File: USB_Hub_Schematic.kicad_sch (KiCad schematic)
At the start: 107 parts, among them J1 USB-C, J2 USB-A, U1 USB2517 Chip, U10 TP, U11 TP, U12 TP, U13 TP, U14 TP, U15 TP, U16 TPS25821, U17 TPS25821, U18 TP, U19 TP, U2 3.3V CONV, U3 MUX, U4 USB to microSD, U5 24AA02, U7 TPS2052B, U9 TP, X3 24MHz Osc

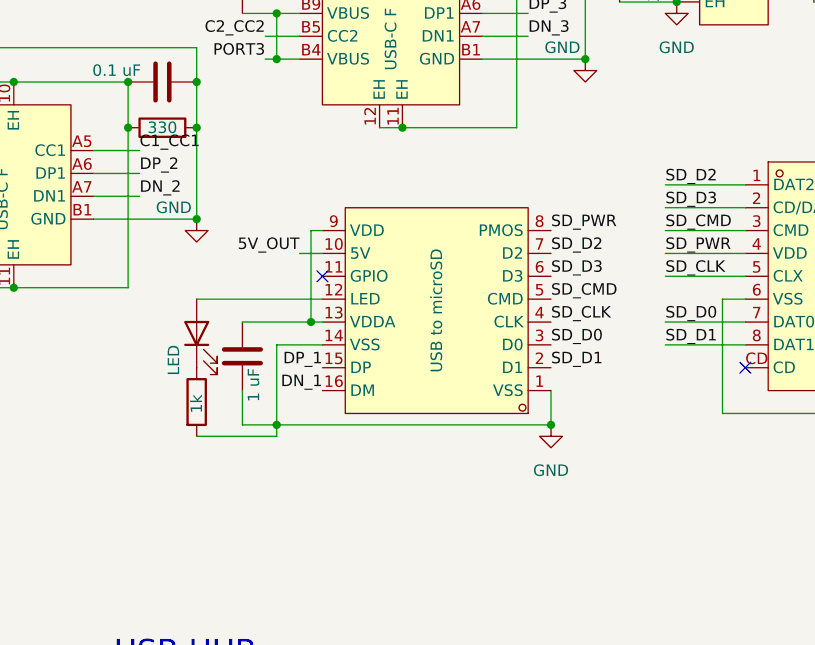
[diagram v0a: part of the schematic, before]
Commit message: PCBWay Order Sent
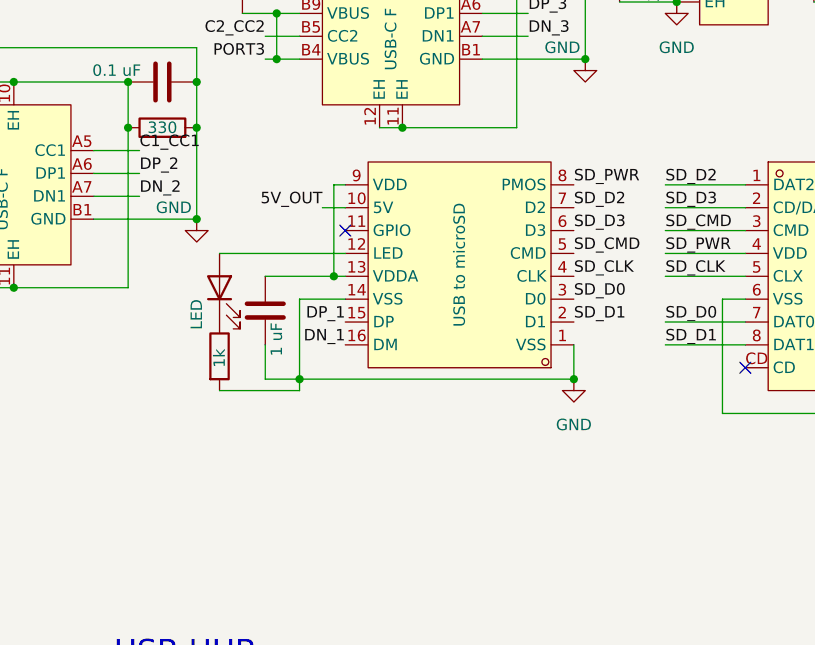
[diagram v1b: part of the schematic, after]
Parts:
- C1, C20, C22, C31, C35, C4, C5: LCSC Part (none) -> C15849
- C12, C13, C17, C3, C33, C38, C39: LCSC Part (none) -> C16780
- C18, C2, C23, C24, C25, C26, C29, C32, C36, C37, C40, C41, C42, C44, C9: LCSC Part (none) -> C1525
- C19, C21, C30, C48: LCSC Part (none) -> C342635
- C28: LCSC Part (none) -> C19666
- C43, C45: LCSC Part (none) -> C15008
- D10, D13, D14, D15, D2: LCSC Part (none) -> C2290
- D11, D12, D16, D17: LCSC Part (none) -> C2286
- R1, R16, R2, R34, R47, R49, R51, R54, R56: LCSC Part (none) -> C25803
- R10, R6: LCSC Part (none) -> C4216
- R11, R13, R15, R27, R28, R29, R3, R38, R4, R41: LCSC Part (none) -> C177337
- R12, R14, R9: LCSC Part (none) -> C861392
- R17: LCSC Part (none) -> C22790
- R21, R23, R30, R31, R5, R52, R53, R55, R57: LCSC Part (none) -> C177649
- R32, R33: LCSC Part (none) -> C23138
- R7: LCSC Part (none) -> C22356449
